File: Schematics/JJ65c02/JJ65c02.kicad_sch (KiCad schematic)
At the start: 21 parts, among them SW1 RESET, U1 74HC00

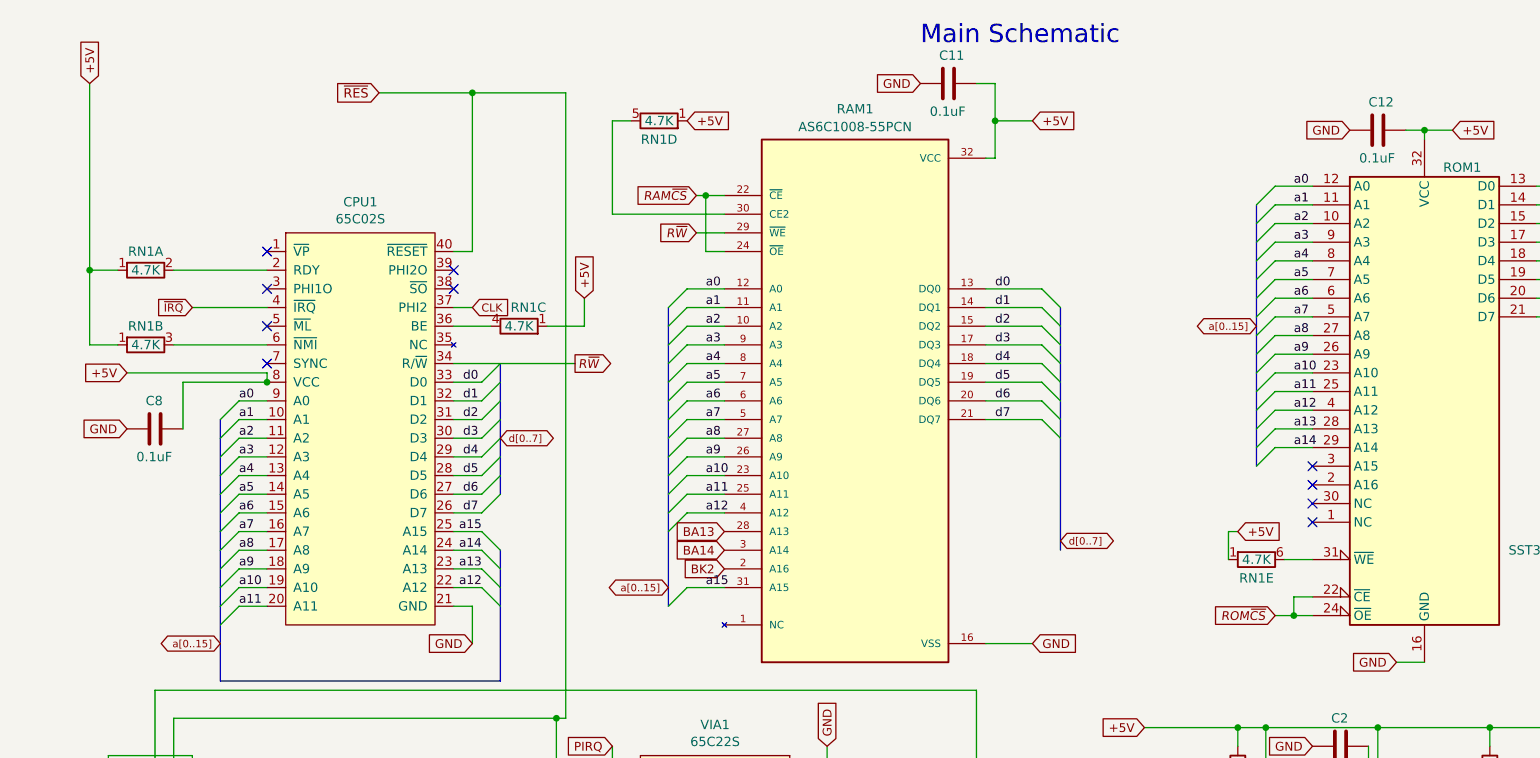
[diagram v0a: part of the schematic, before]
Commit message: More work on rp2040-version2
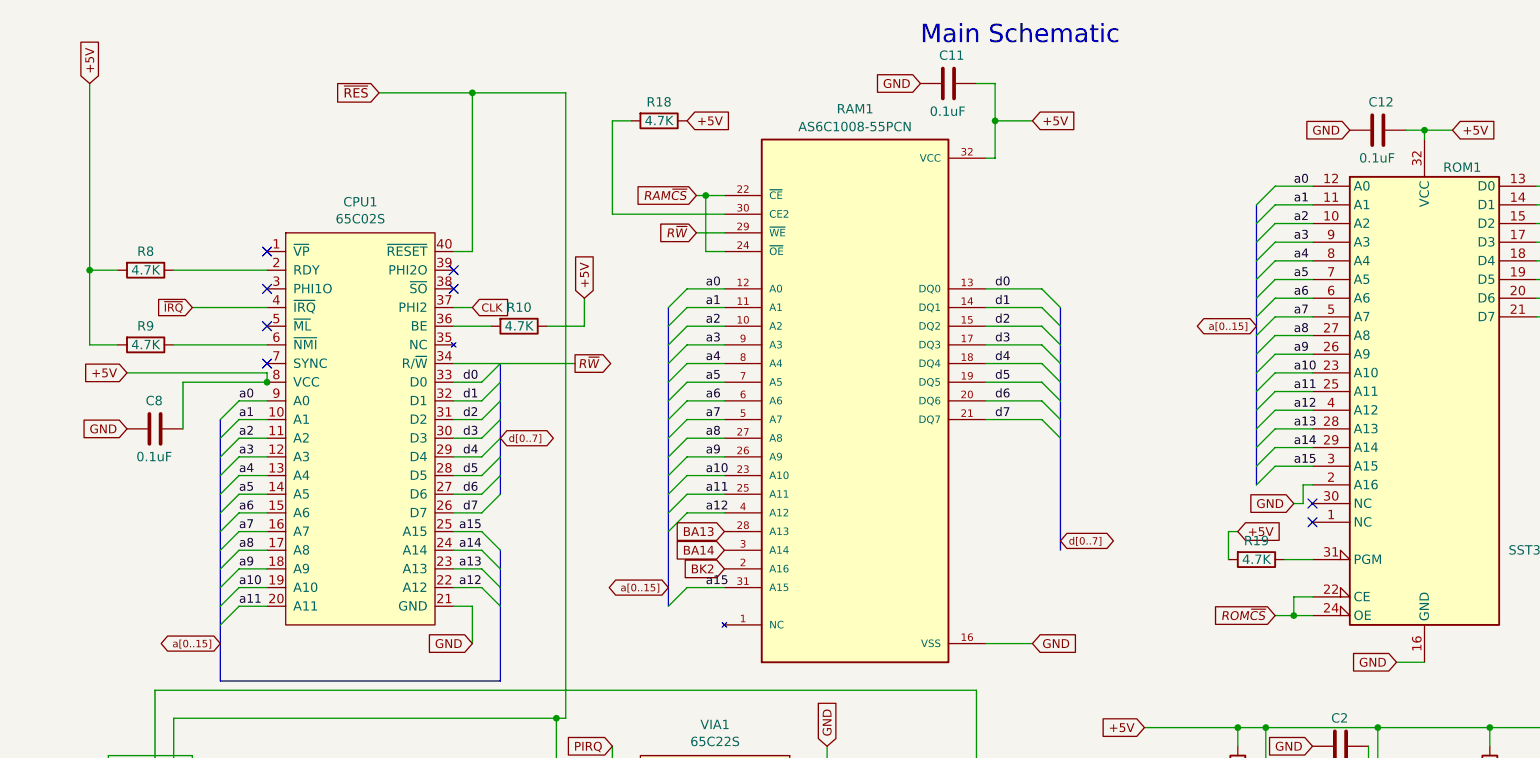
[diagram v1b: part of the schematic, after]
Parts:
- removed RN1: 4.7K, Resistor_THT:R_Array_SIP6, symbol Device:R_Network06_Split
- added R10, R18, R19, R8, R9: 4.7K, Resistor_THT:R_Axial_DIN0207_L6.3mm_D2.5mm_P7.62mm_Horizontal, symbol Device:R
- RAM1: footprint JJ65c02:DIP1524W45P254L4191H419Q32 -> DIP1524W45P254L4191H419Q32
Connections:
- net +5V: now also R10.1, R18.1, R19.2, R8.2, R9.2
- net GND: now also ROM1.2 (A16)
- net a15: now also ROM1.3 (A15)
- net at CPU1.2 (RDY): now also R8.1
- net at CPU1.36 (BE): now also R10.2
- net at CPU1.6 (~{NMI}): now also R9.1
- net at RAM1.30 (CE2): now also R18.2
- net at ROM1.31 (PGM): now also R19.1
- no-connect marks 24 -> 22
